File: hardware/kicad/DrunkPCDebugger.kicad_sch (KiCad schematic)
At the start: 104 parts, among them Q1 AO3400A, Q2 AO3401A, Q3 AO3401A, Q4 AO3400A, SW2 TS3643TP, SW3 TS3643TP, U1 SN74LVC4245APWR, U10 A-SC6302R6AGHC-A03-2T, U11 SN74LVC3G07DCTR, U2 STM32H723VET6, U3 SN74LVC4245APWR, U4 SN74LVC4245APWR, U5 X6521FV-2X27-C85D32, U6 AMS1117-3_3, U7 SN74LVC4245APWR, U8 SN74LVC3G17DCTR, X1 X322525MOB4SI

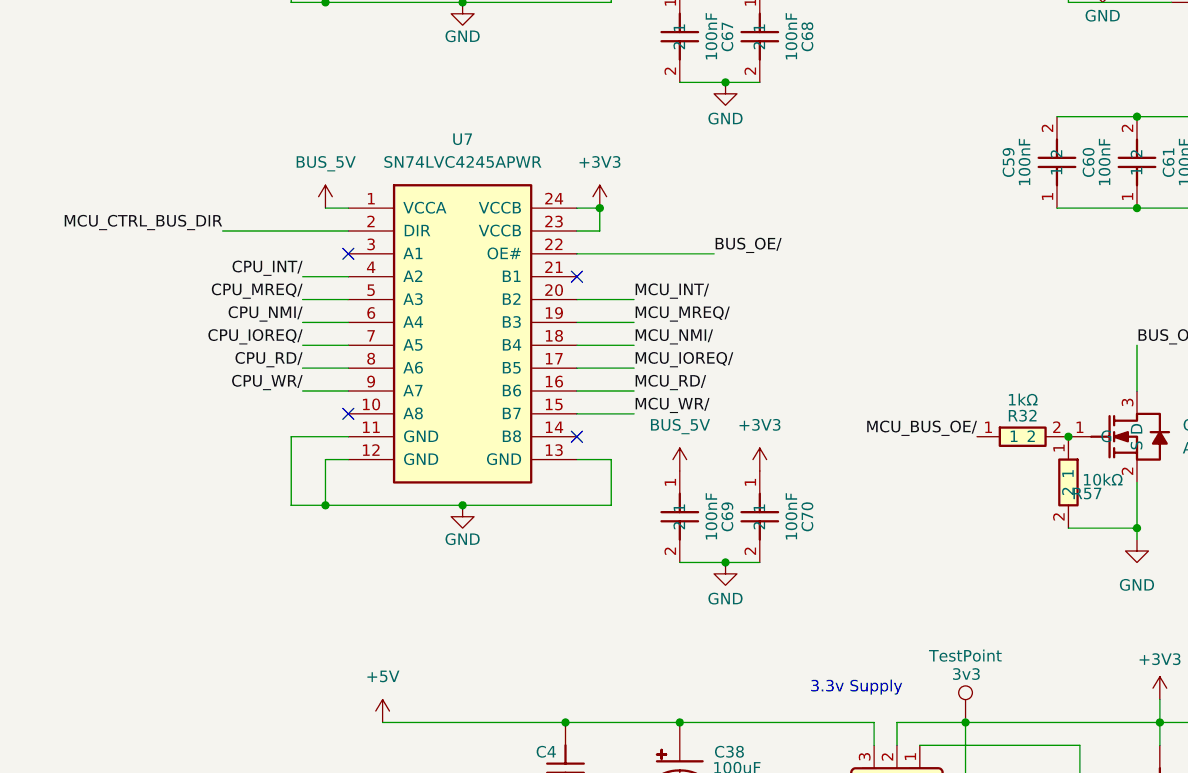
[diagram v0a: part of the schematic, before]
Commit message: Pcb production
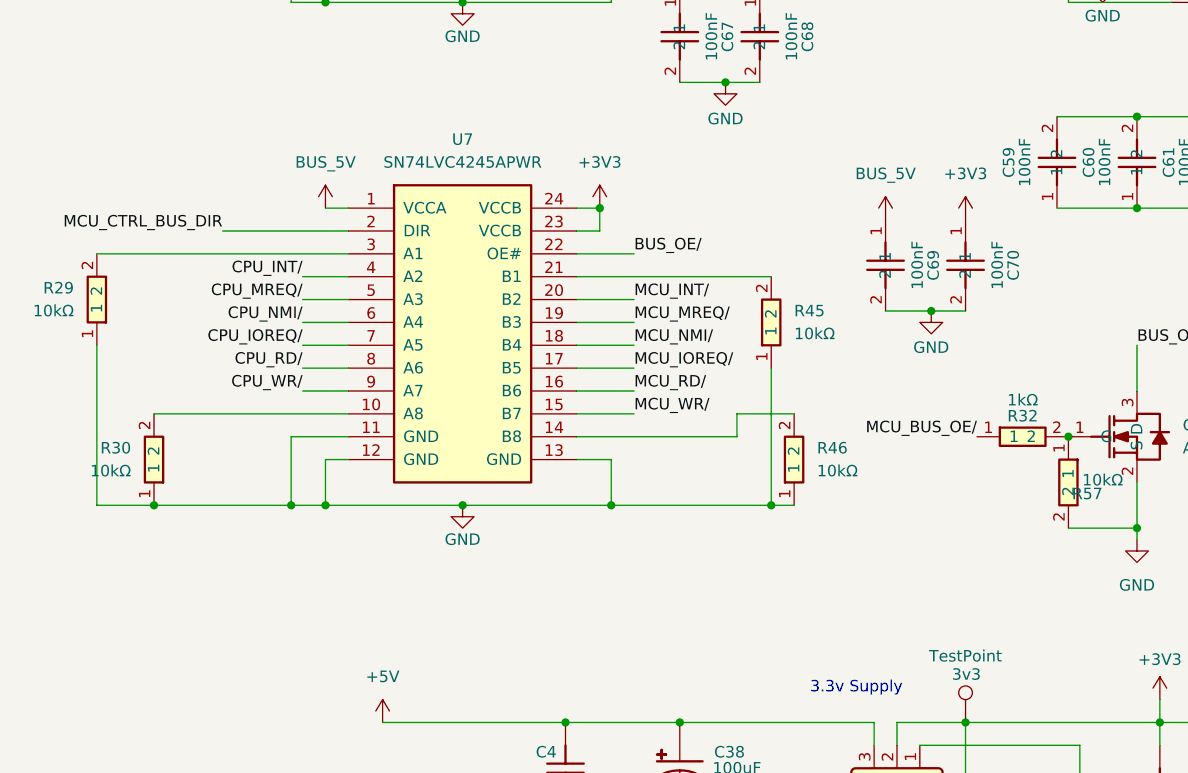
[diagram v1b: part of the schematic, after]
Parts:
- added R29, R30, R45, R46: 10kΩ, Resistor_SMD:R_0603_1608Metric, symbol JLCImport:0603WAF1002T5E
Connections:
- net GND: now also R29.1, R30.1, R45.1, R46.1
- net at U7.10 (A8): now also R30.2
- net at U7.14 (B8): now also R46.2
- net at U7.21 (B1): now also R45.2
- net at U7.3 (A1): now also R29.2
- no-connect marks 39 -> 35
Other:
- moved on the sheet: C69, C70
